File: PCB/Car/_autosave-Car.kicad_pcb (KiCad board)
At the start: 2 copper layers, 70 x 64 mm, 12 parts, among them J1 L1, J10 FL2, J11 FLT, J2 L2, J3 R1, J4 R2, J5 R1+2, J6 L1+2, J7 Conn_01x03, J8 pi zero 2 w, J9 FL1, U3 YAAJ_DCDC_StepDown_LM2596

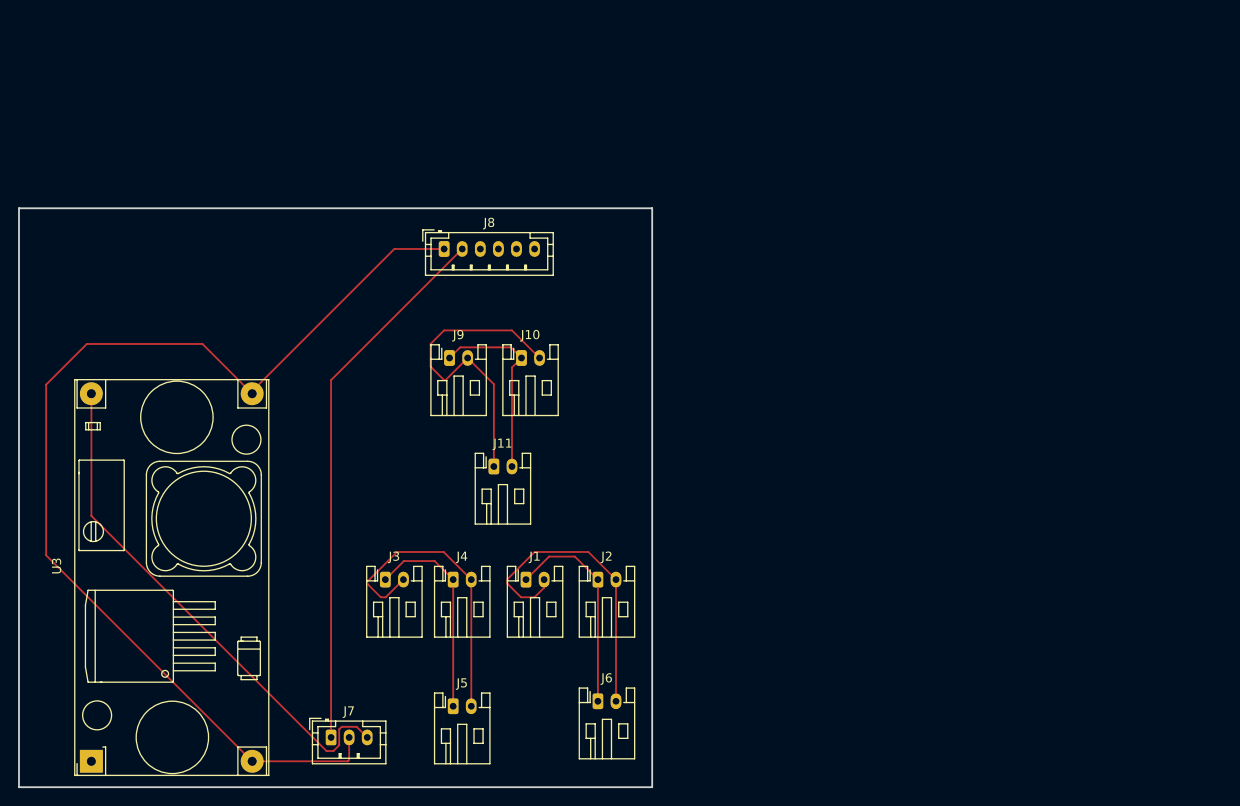
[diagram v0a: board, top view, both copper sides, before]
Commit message: updated CAD + PCB
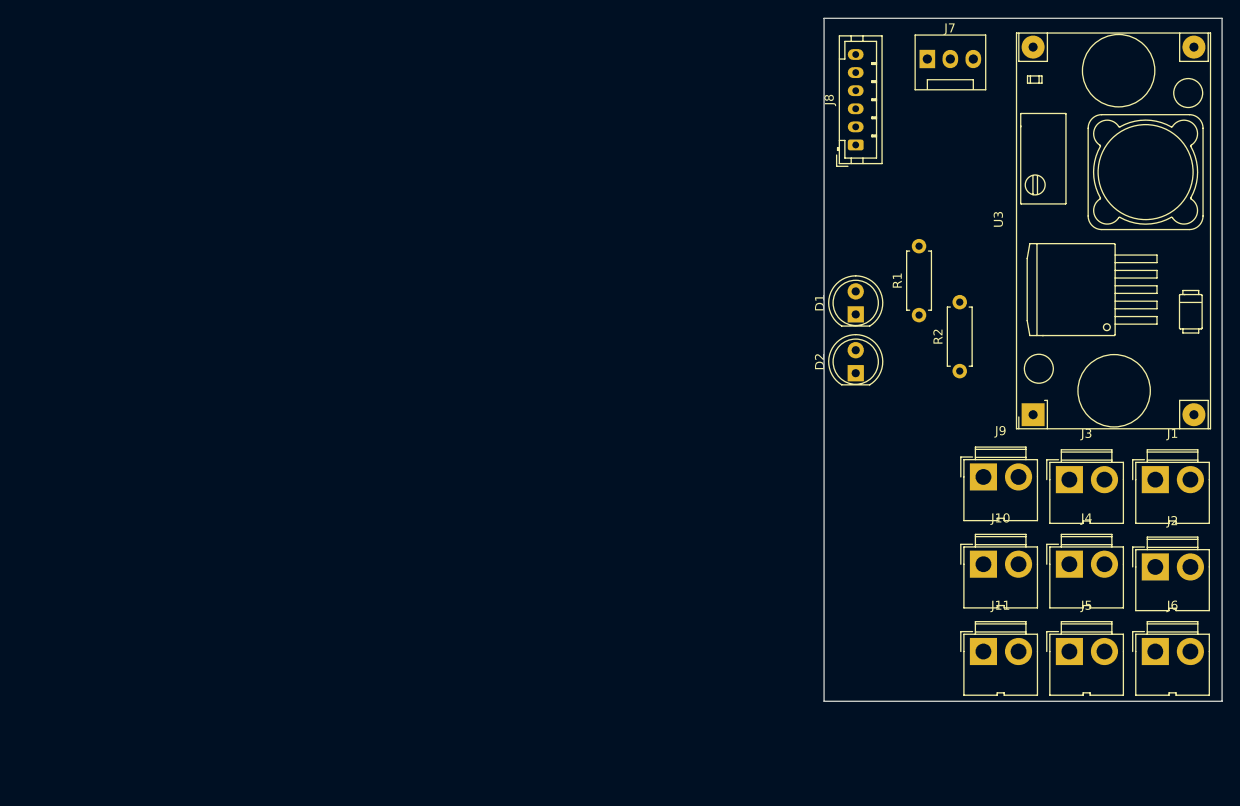
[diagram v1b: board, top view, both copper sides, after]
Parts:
- added D1: LED, LED_THT:LED_D5.0mm, F.Cu at (192.5, 95.7)
- added D2: LED, LED_THT:LED_D5.0mm, F.Cu at (192.5, 102.2)
- added R1: 220ohms, Resistor_THT:R_Axial_DIN0207_L6.3mm_D2.5mm_P7.62mm_Horizontal, F.Cu at (199.5, 95.8)
- added R2: 220ohms, Resistor_THT:R_Axial_DIN0207_L6.3mm_D2.5mm_P7.62mm_Horizontal, F.Cu at (204.0, 102.0)
- J1, J10, J11, J2, J3, J4, J5, J6, J9: footprint Connector_JST:JST_PH_S2B-PH-K_1x02_P2.00mm_Horizontal -> Connector:JWT_A3963_1x02_P3.96mm_Vertical
- J7: footprint Connector_JST:JST_PH_B3B-PH-K_1x03_P2.00mm_Vertical -> Connector:FanPinHeader_1x03_P2.54mm_Vertical
- moved U3 110.9 mm to (212.1, 106.8)
- moved J7 99.9 mm to (200.4, 67.5)
- moved J3 76.4 mm to (216.1, 114.0)
- moved J1 70.4 mm to (225.6, 114.0)
- moved J5 68.4 mm to (216.1, 133.0)
- moved J4 68.1 mm to (216.1, 123.3)
- moved J6 61.9 mm to (225.6, 133.0)
- moved J2 61.6 mm to (225.6, 123.7)
- moved J9 60.5 mm to (206.6, 113.7)
- moved J11 57.9 mm to (206.6, 133.0)
- moved J10 55.9 mm to (206.6, 123.3)
- moved J8 46.9 mm to (192.5, 77.0), turned to 90 degrees
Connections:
- net +6V renamed +6.5V
- J11 pad 1: Net-(J10-Pin_2) -> Net-(J10-Pin_1)
- J11 pad 2: Net-(J10-Pin_1) -> Net-(J10-Pin_2)
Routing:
- net GND: track 119.3 -> 0.00 mm
- net +5V: track 60.0 -> 0.00 mm
- net +6.5V: track 57.4 -> 0.00 mm
- net Net-(J10-Pin_2): track 35.4 -> 0.00 mm
- net Net-(J1-Pin_2): track 34.5 -> 0.00 mm
- net Net-(J3-Pin_2): track 33.8 -> 0.00 mm
- net Net-(J1-Pin_1): track 23.5 -> 0.00 mm
- net Net-(J3-Pin_1): track 23.2 -> 0.00 mm
- net Net-(J10-Pin_1): track 21.4 -> 0.00 mm
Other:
- board size 70 x 64 mm -> 44 x 75.5 mm
